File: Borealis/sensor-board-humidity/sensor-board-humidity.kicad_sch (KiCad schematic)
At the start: 3 parts, among them J1 Conn_01x06_Pin, J2 Conn_01x07_Pin

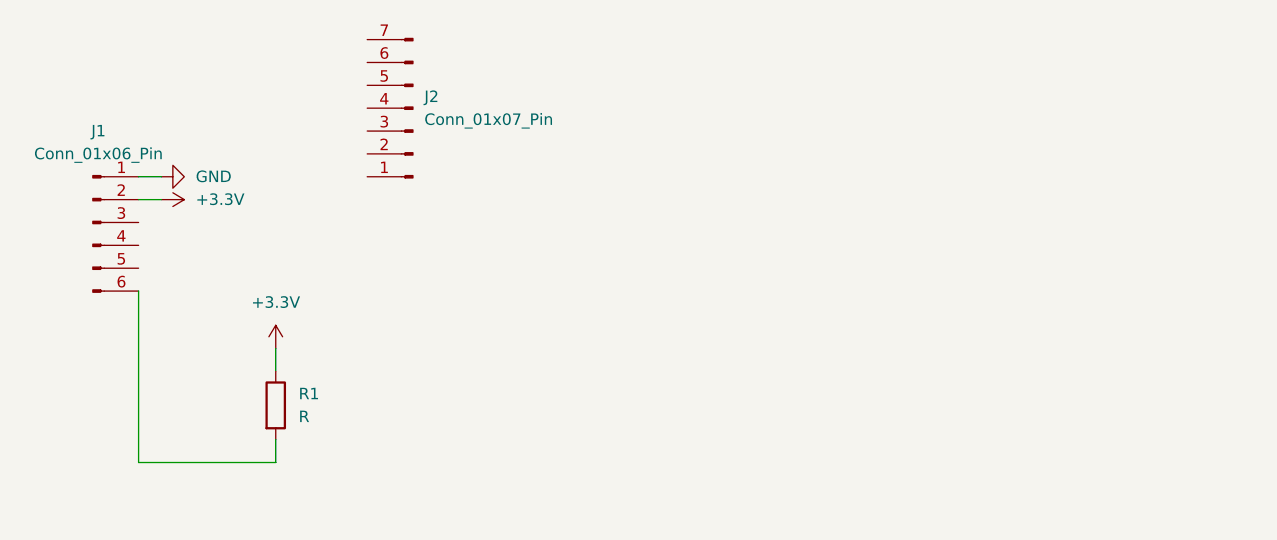
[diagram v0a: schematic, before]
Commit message: Updating changes
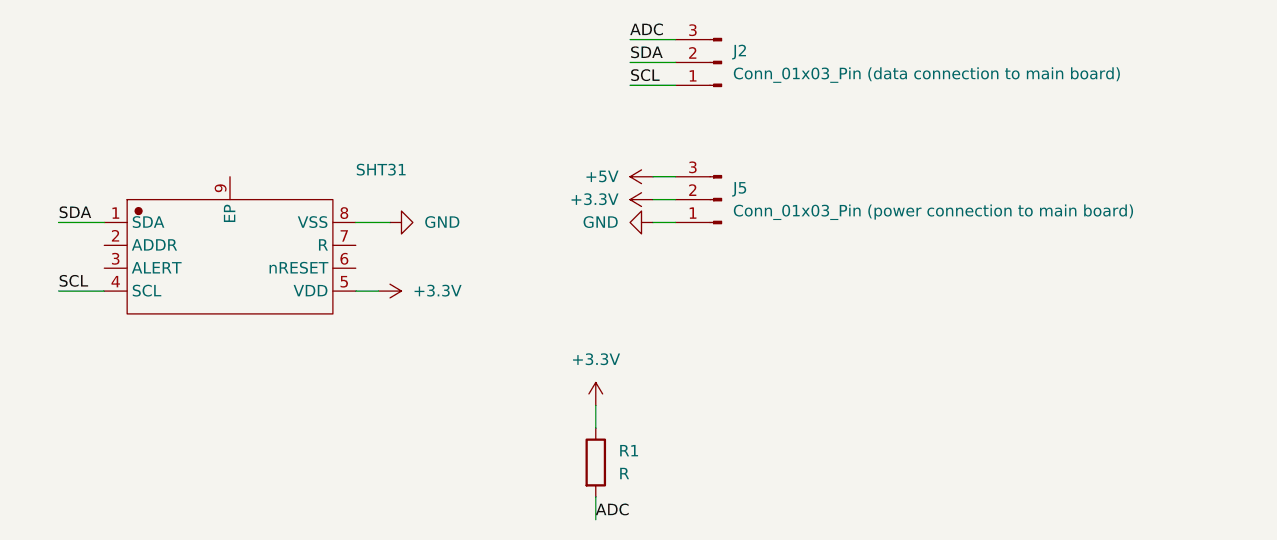
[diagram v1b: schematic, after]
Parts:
- removed J1: Conn_01x06_Pin, symbol Connector:Conn_01x06_Pin
- removed J2: Conn_01x07_Pin, symbol Connector:Conn_01x07_Pin
- added J2: Conn_01x03_Pin (data connection to main board), batteryholder:1x03 2.3 pitch, symbol Connector:Conn_01x03_Pin
- added J5: Conn_01x03_Pin (power connection to main board), batteryholder:1x03 2.3 pitch, symbol Connector:Conn_01x03_Pin
- added SHT31: ~, batteryholder:sht31-footprint, symbol SHT31-DIS-F2.5KS_2025-12-25-altium-import:root_0_SHT31-DIS-F2.5KS_
- R1: footprint (none) -> OptoDevice:R_LDR_4.9x4.2mm_P2.54mm_Vertical
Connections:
- net +3.3V: now also J5.2 (Pin_2), SHT31.5 (VDD)
- net GND: now also J5.1 (Pin_1), SHT31.8 (VSS)
- net ADC: now reaches R1.2
- net ADC: now also J2.3 (Pin_3)
- new net +5V: J5.3 (Pin_3)
- new net SCL: J2.1 (Pin_1), SHT31.4 (SCL)
- new net SDA: J2.2 (Pin_2), SHT31.1 (SDA)
